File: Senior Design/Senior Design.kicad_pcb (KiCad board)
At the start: 2 copper layers, 27 parts, among them U1 Raspberry_Pi_Zero_W, U2 AP1509, U3 TPA2005D1DRB, U4 ADC1210S21

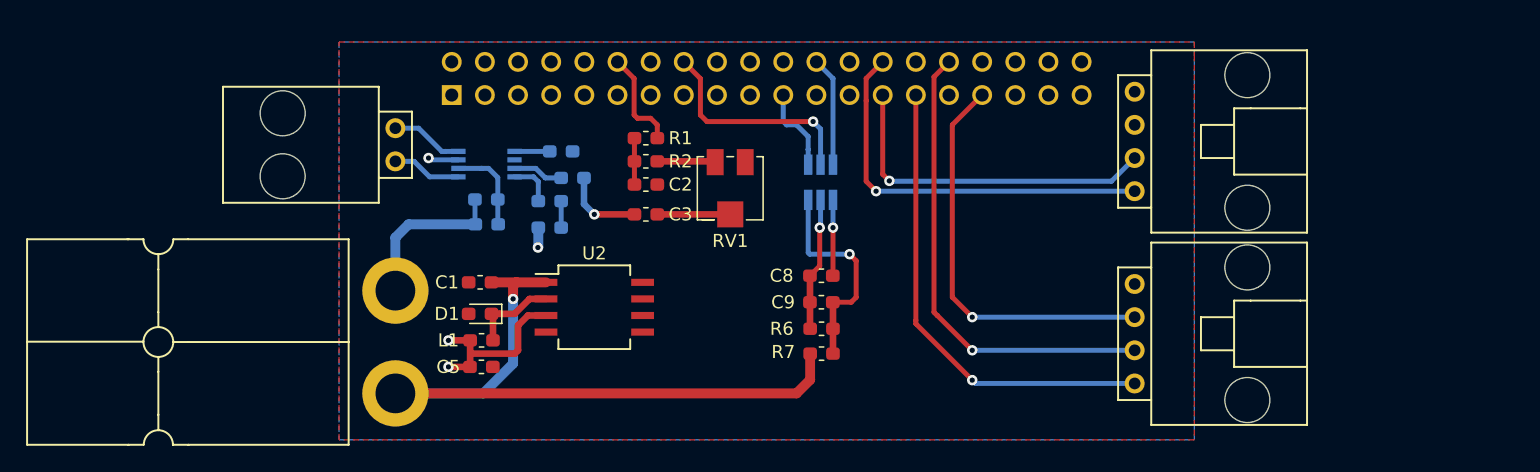
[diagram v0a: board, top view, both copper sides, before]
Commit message: update
ddds
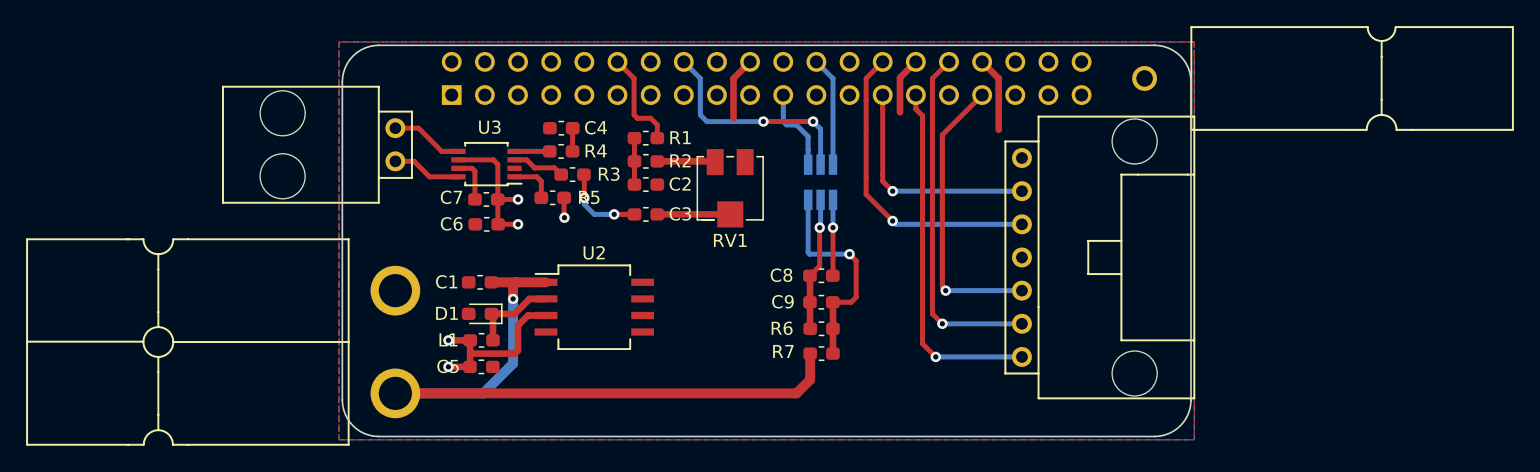
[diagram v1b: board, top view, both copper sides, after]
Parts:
- C1, C5: value CP1 -> 10uF
- C3: value 1u -> 1uF
- C4, C6, C7: value 1u -> 1uF; moved to F.Cu
- C8: value C_Small -> 1uF
- C9: value C_Small -> 0.1uF
- Conn1: value Molex_SL_04 -> Molex_SL_07; footprint MRDT_Connectors:MOLEX_SL_04_Horizontal -> MRDT_Connectors:MOLEX_SL_07_Horizontal
- Conn2: value Molex_SL_04 -> AndersonPP; footprint MRDT_Connectors:MOLEX_SL_04_Horizontal -> MRDT_Connectors:Anderson_1_Horizontal
- R3, R4, R5, U3: moved to F.Cu
- moved Conn1 13.0 mm to (166.6, 70.4)
- moved C4 7.67 mm to (131.3, 68.1)
- moved R4 3.91 mm to (131.3, 69.8)
- moved R5 3.61 mm to (130.7, 73.4)
- moved Conn2 1.39 mm to (176.0, 64.1), turned to 180 degrees
- moved R3 0.25 mm to (132.2, 71.6)
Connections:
- C5 pad 1: +3V3 -> +5V
- C6 pad 2: +3V3 -> +5V
- C7 pad 2: +3V3 -> +5V
- C8 pad 1: +3V3 -> +5V
- Conn1 pad 2: LED_3 -> IMU_SDA
- Conn1 pad 3: LED_2 -> IMU_SCL
- Conn1 pad 4: LED_1 -> +5V
- Conn2 pad 1: GND -> (no net)
- Conn3 pad 1: Speak_OUT+ -> Speak_OUT-
- Conn3 pad 2: Speak_OUT- -> Speak_OUT+
- L1 pad 2: +3V3 -> +5V
- R5 pad 2: +3V3 -> +5V
- U1 pad 2: Net-(U1-Pad2) -> +5V
- U1 pad 4: Net-(U1-Pad4) -> +5V
- U2 pad 3: +3V3 -> +5V
- U3 pad 6: +3V3 -> +5V
- U4 pad 1: +3V3 -> +5V
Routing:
- net +5V: track 0.00 -> 31.7 mm, vias 0 -> 6
- net +3V3: track 26.3 -> 0.00 mm, vias 3 -> 0
- net LED_2: track 36.2 -> 26.7 mm
- net LED_1: track 36.5 -> 27.3 mm
- net LED_3: track 31.0 -> 22.2 mm
- net IMU_SDA: track 26.3 -> 17.6 mm
- net IMU_SCL: track 30.6 -> 23.6 mm
- net GND: track 16.4 -> 18.5 mm, vias 2 -> 0
- net Net-(R5-Pad1): track 2.70 -> 3.46 mm
- net Speak_OUT-: track 5.92 -> 5.32 mm
- net Net-(R4-Pad1): track 3.22 -> 2.70 mm
- net Net-(C3-Pad1): vias 1 -> 2
- net AD_Vout: vias 1 -> 2
- added copper zone on B.Cu, net +5V
- removed copper zone on B.Cu, net +3V3
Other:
- board outline added: 65 x 30 mm
